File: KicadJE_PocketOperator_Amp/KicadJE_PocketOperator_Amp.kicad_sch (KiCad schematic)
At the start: 10 parts, among them J101 AudioJack3_Ground, J102 AudioJack3_Ground, J103 AudioJack3_Ground

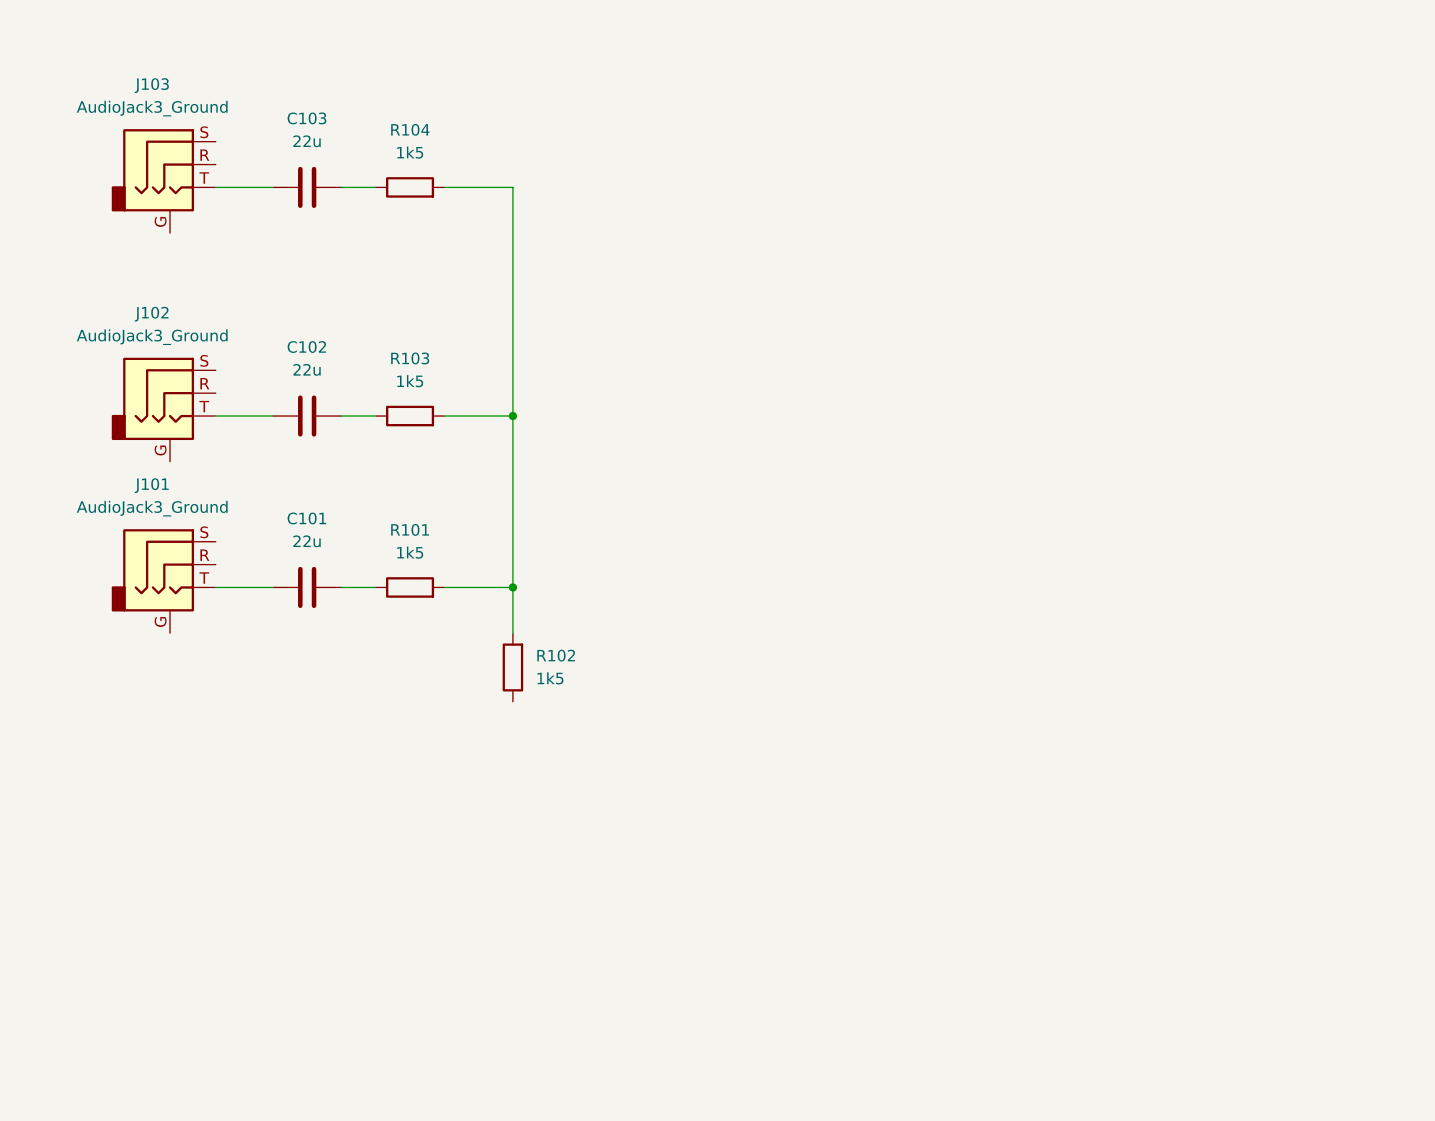
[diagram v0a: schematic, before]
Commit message: Initial base sch
Initial base sch
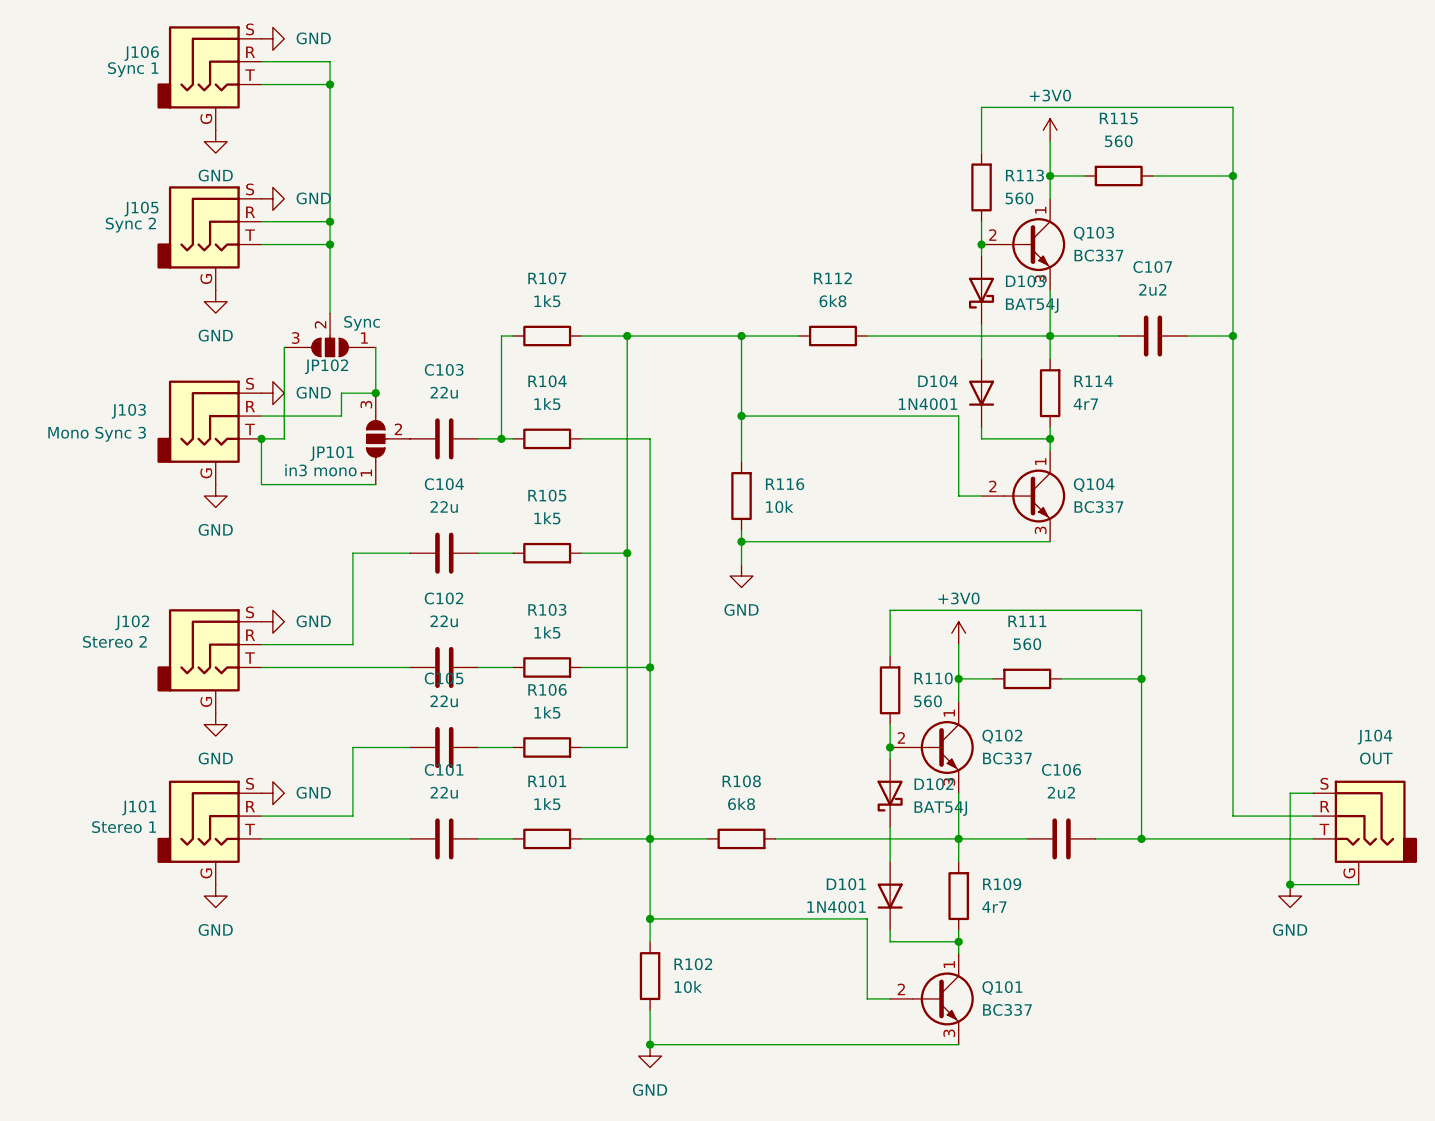
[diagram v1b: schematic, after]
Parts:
- added C104, C105: 22u, symbol Device:C
- added C106, C107: 2u2, symbol Device:C
- added D101, D104: 1N4001, Diode_THT:D_DO-41_SOD81_P10.16mm_Horizontal, symbol Diode:1N4001
- added D102, D103: BAT54J, Diode_SMD:D_SOD-323F, symbol Diode:BAT54J
- added J104: OUT, symbol Connector_Audio:AudioJack3_Ground
- added J105: Sync 2, symbol Connector_Audio:AudioJack3_Ground
- added J106: Sync 1, symbol Connector_Audio:AudioJack3_Ground
- added JP101: in3 mono, symbol Jumper:SolderJumper_3_Open
- added JP102: Sync, symbol Jumper:SolderJumper_3_Open
- added Q101, Q102, Q103, Q104: BC337, Package_TO_SOT_THT:TO-92_Inline, symbol Transistor_BJT:BC337
- added R105, R106, R107: 1k5, symbol Device:R
- added R108, R112: 6k8, symbol Device:R
- added R109, R114: 4r7, symbol Device:R
- added R110, R111, R113, R115: 560, symbol Device:R
- added R116: 10k, symbol Device:R
- J101: value AudioJack3_Ground -> Stereo 1
- J102: value AudioJack3_Ground -> Stereo 2
- J103: value AudioJack3_Ground -> Mono Sync 3
- R102: value 1k5 -> 10k
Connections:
- net GND: now reaches R102.1
- net GND: now also J101.G, J101.S, J102.G, J102.S, J103.G, J103.S, J104.G, J104.S, J105.G, J105.S, J106.G, J106.S, Q101.3 (E), Q104.3 (E), R116.1
- net at R101.2, R102.2, R103.2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: now also Q101.2 (B), R108.1
- net at J101.R: now also C105.1
- net at C103.1: now also JP101.2 (C); no longer J103.T
- net at C103.2, R104.1: now also R107.1
- net at J103.R: now also JP101.3 (B), JP102.1 (A)
- net at J102.R: now also C104.1
- new net: D104.1 (K), Q104.1 (C), R114.1
- new net: Q104.2 (B), R105.2, R106.2, R107.2, R112.1, R116.2
- new net: D102.2 (A), Q102.2 (B), R110.1
- new net: C106.1, Q102.3 (E), R108.2, R109.2
- new net: D101.1 (K), Q101.1 (C), R109.1
- new net: D103.1 (K), D104.2 (A)
- new net: D103.2 (A), Q103.2 (B), R113.1
- new net: C107.1, Q103.3 (E), R112.2, R114.2
- new net: C107.2, J104.R, R113.2, R115.1
- new net: J105.R, J105.T, J106.R, J106.T, JP102.2 (C)
- new net: C106.2, J104.T, R110.2, R111.1
- new net: D101.2 (A), D102.1 (K)
- new net: C105.2, R106.1
- new net: J103.T, JP101.1 (A), JP102.3 (B)
- new net: C104.2, R105.1
- new net +3V0: Q102.1 (C), Q103.1 (C), R111.2, R115.2
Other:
- moved on the sheet: C101, C102, C103, J101, J102, J103, R101, R102, R103, R104
